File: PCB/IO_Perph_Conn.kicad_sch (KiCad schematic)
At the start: 18 parts, among them J2 Conn_02x06_Odd_Even, U4 STM32MP157FABx, Y601 NX2012SA-32.768K

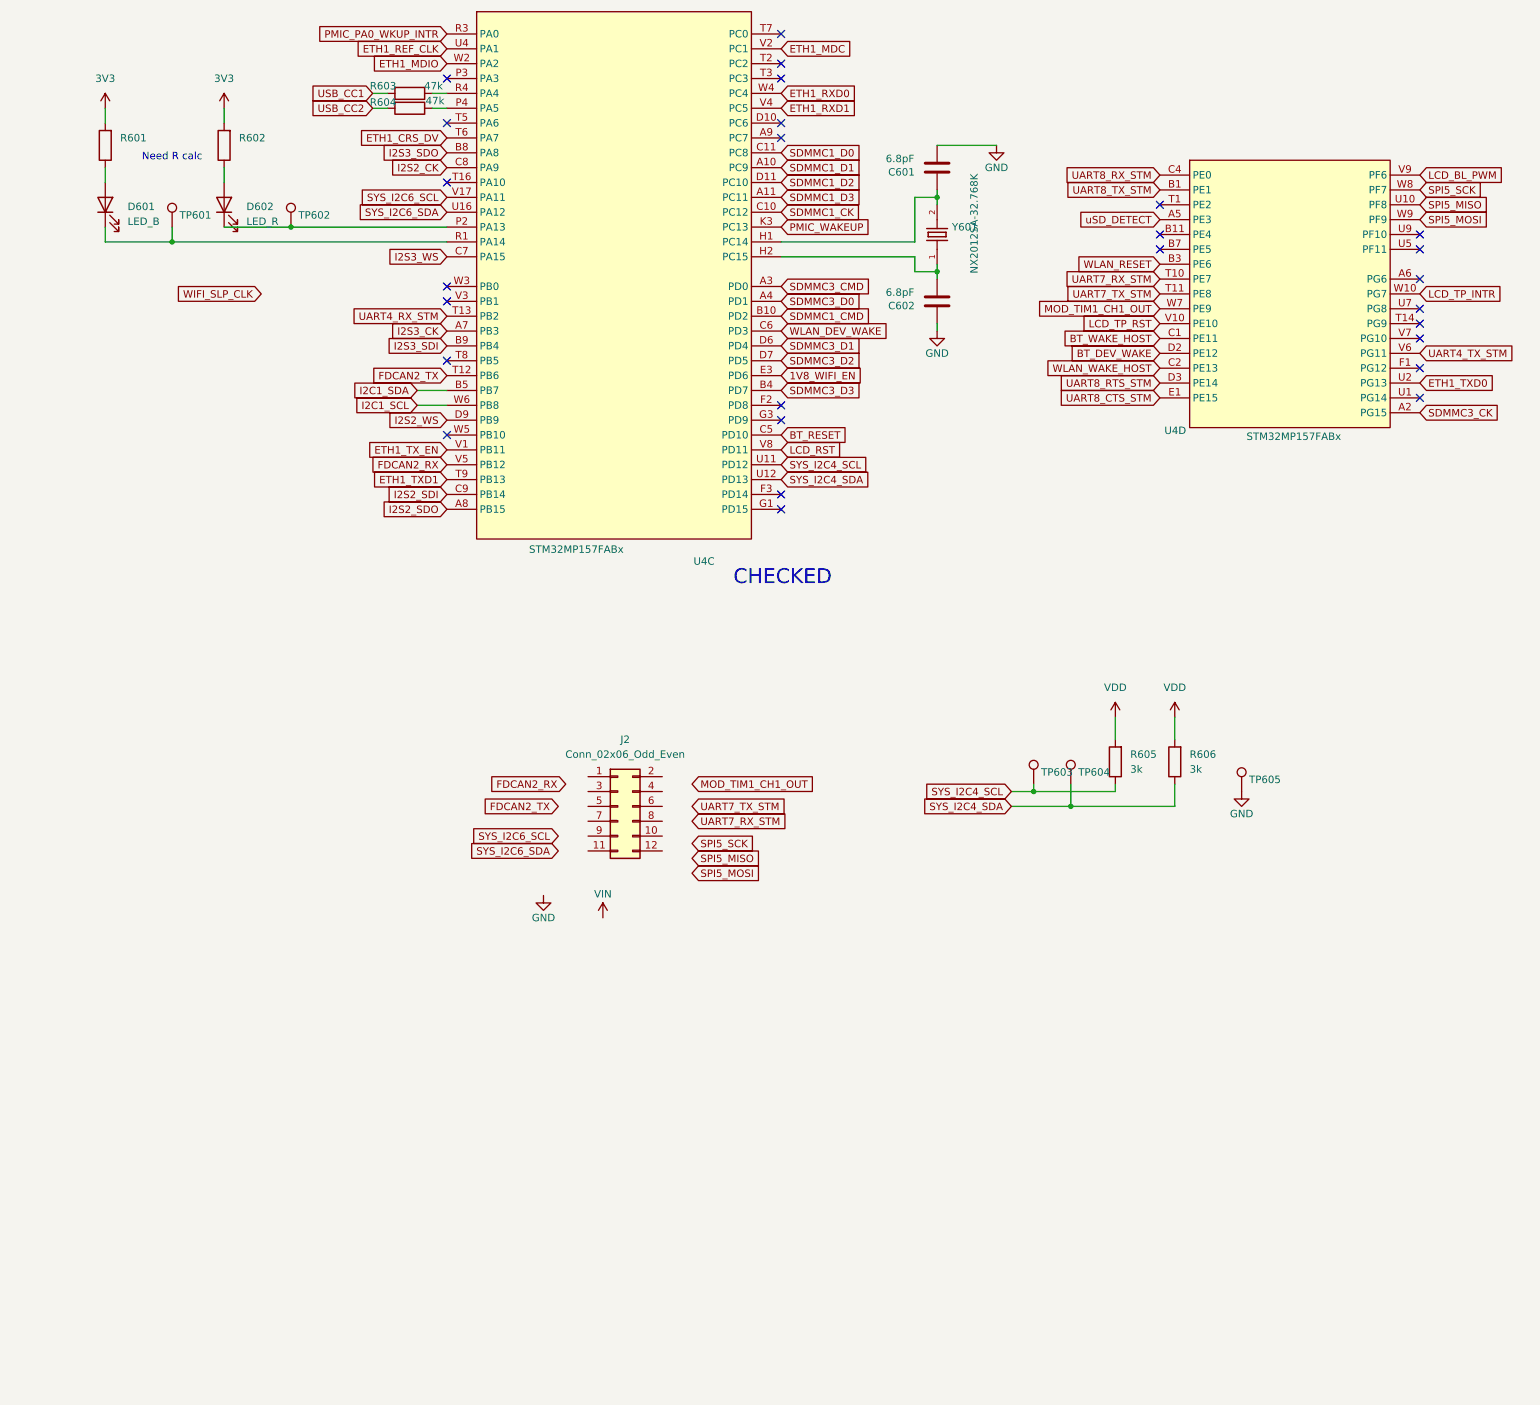
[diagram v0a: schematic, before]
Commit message: UPDATE
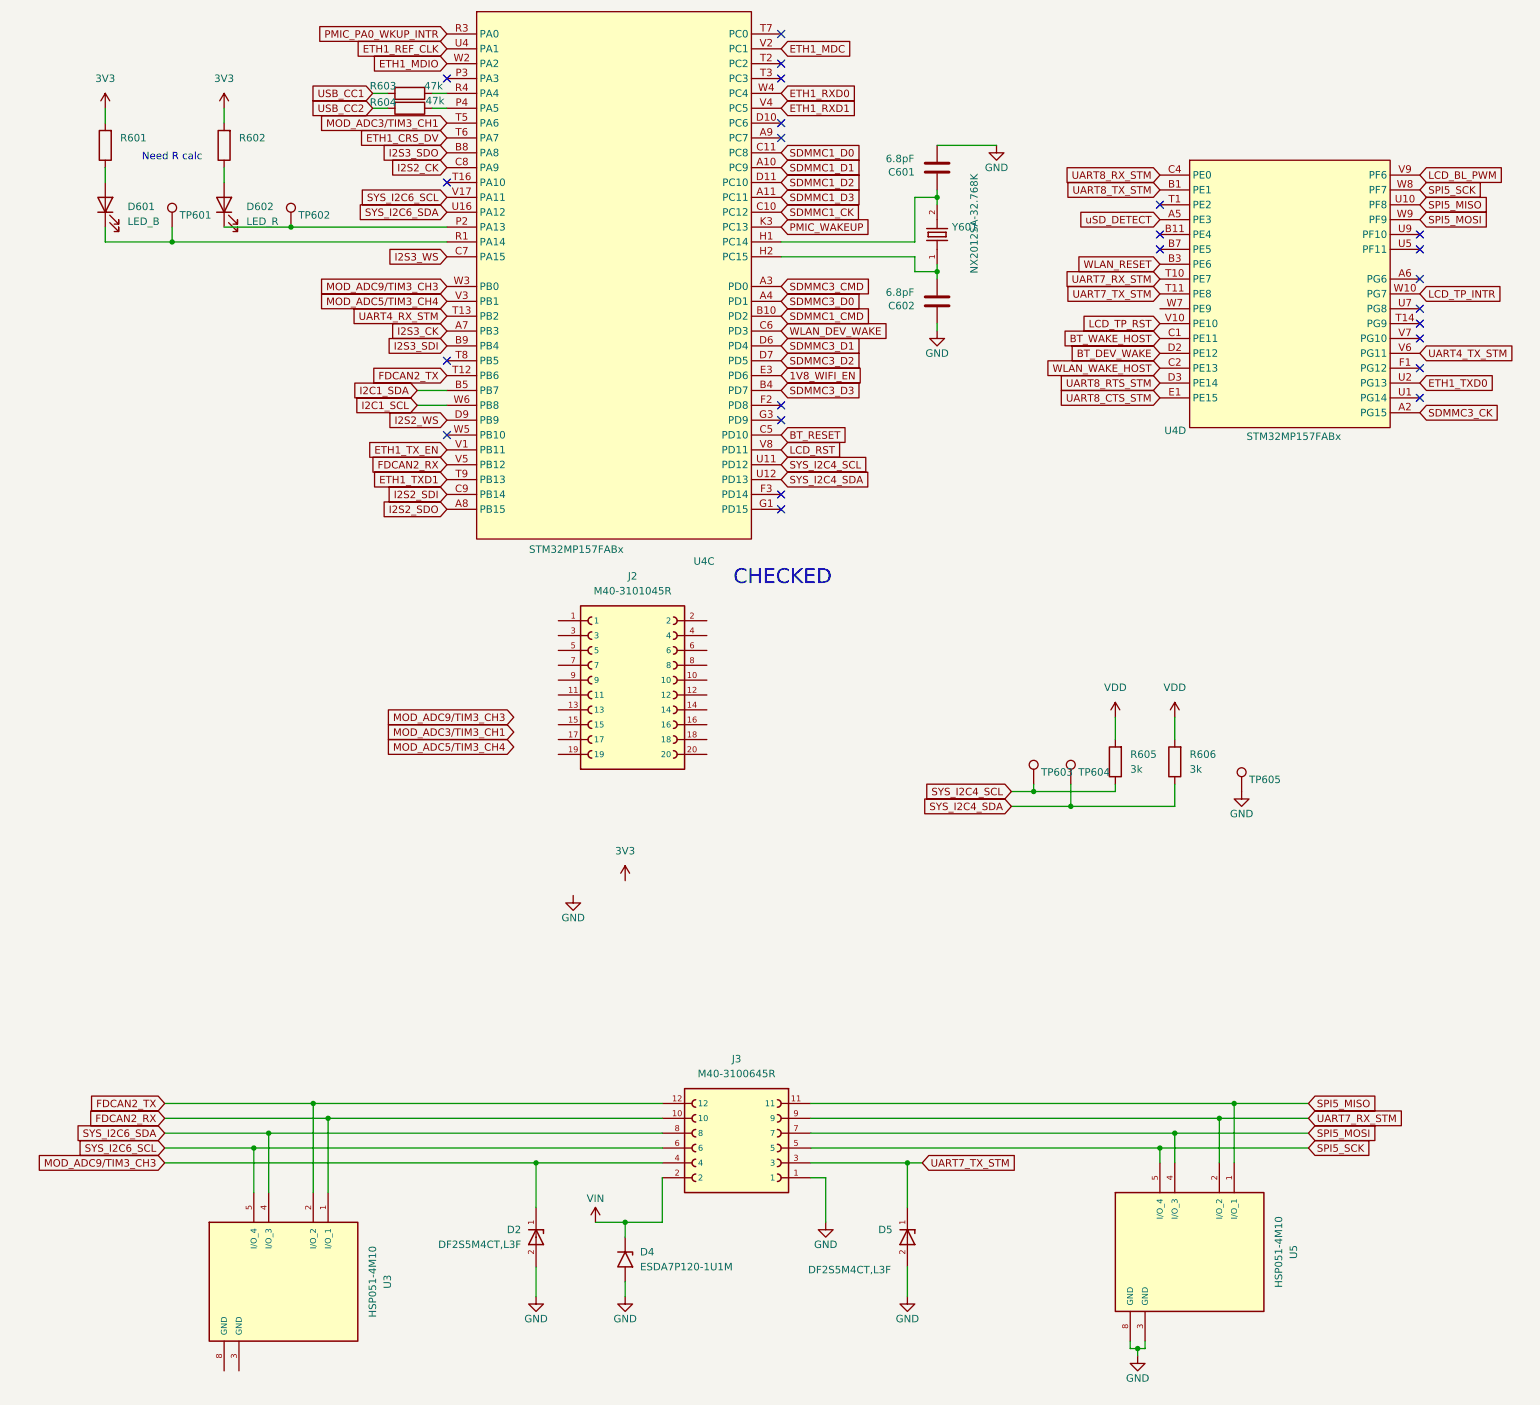
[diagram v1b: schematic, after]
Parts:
- removed J2: Conn_02x06_Odd_Even, Connector_PinHeader_1.00mm:PinHeader_2x06_P1.00mm_Vertical_SMD, symbol Connector_Generic:Conn_02x06_Odd_Even
- added D2, D5: DF2S5M4CT,L3F, Diode_SMD:D_SOD-882, symbol PTVS3V3S1UR:PTVS3V3S1UR
- added D4: ESDA7P120-1U1M, lib:DIODE_ESDA7P120-1U1M_STM, symbol Diode:SMAJ5.0A
- added J2: M40-3101045R, lib:HARWIN_M40-3101045R, symbol M40-3101045R:M40-3101045R
- added J3: M40-3100645R, lib:HARWIN_M40-3100645R, symbol M40-3100645R:M40-3100645R
- added U3, U5: HSP051-4M10, lib:IC_HSP051-4M10, symbol HSP051-4M10:HSP051-4M10
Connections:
- net FDCAN2_RX: now also J3.10, U3.1 (I/O_1), U3.10 (NC)
- net FDCAN2_TX: now also J3.12, U3.2 (I/O_2), U3.9 (NC)
- net GND: now also D2.2, D4.2 (A2), D5.2, J3.1, U5.3 (GND), U5.8 (GND)
- net SPI5_MISO: now also J3.11, U5.1 (I/O_1), U5.10 (NC)
- net SPI5_MOSI: now also J3.7, U5.4 (I/O_3), U5.7 (NC)
- net SPI5_SCK: now also J3.5, U5.5 (I/O_4), U5.6 (NC)
- net SYS_I2C6_SCL: now also J3.6, U3.5 (I/O_4), U3.6 (NC)
- net SYS_I2C6_SDA: now also J3.8, U3.4 (I/O_3), U3.7 (NC)
- net UART7_RX_STM: now also J3.9, U5.2 (I/O_2), U5.9 (NC)
- net UART7_TX_STM: now also D5.1, J3.3
- net VIN: now also D4.1 (A1), J3.2
- net MOD_ADC3/TIM3_CH1: now reaches U4.T5 (PA6)
- net MOD_ADC5/TIM3_CH4: now reaches U4.V3 (PB1)
- net MOD_ADC9/TIM3_CH3: now reaches U4.W3 (PB0)
- net MOD_ADC9/TIM3_CH3: now also D2.1, J3.4
- net MOD_TIM1_CH1_OUT: no longer names the net of U4.W7 (PE9)
- no-connect marks 27 -> 24

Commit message: UPDATE
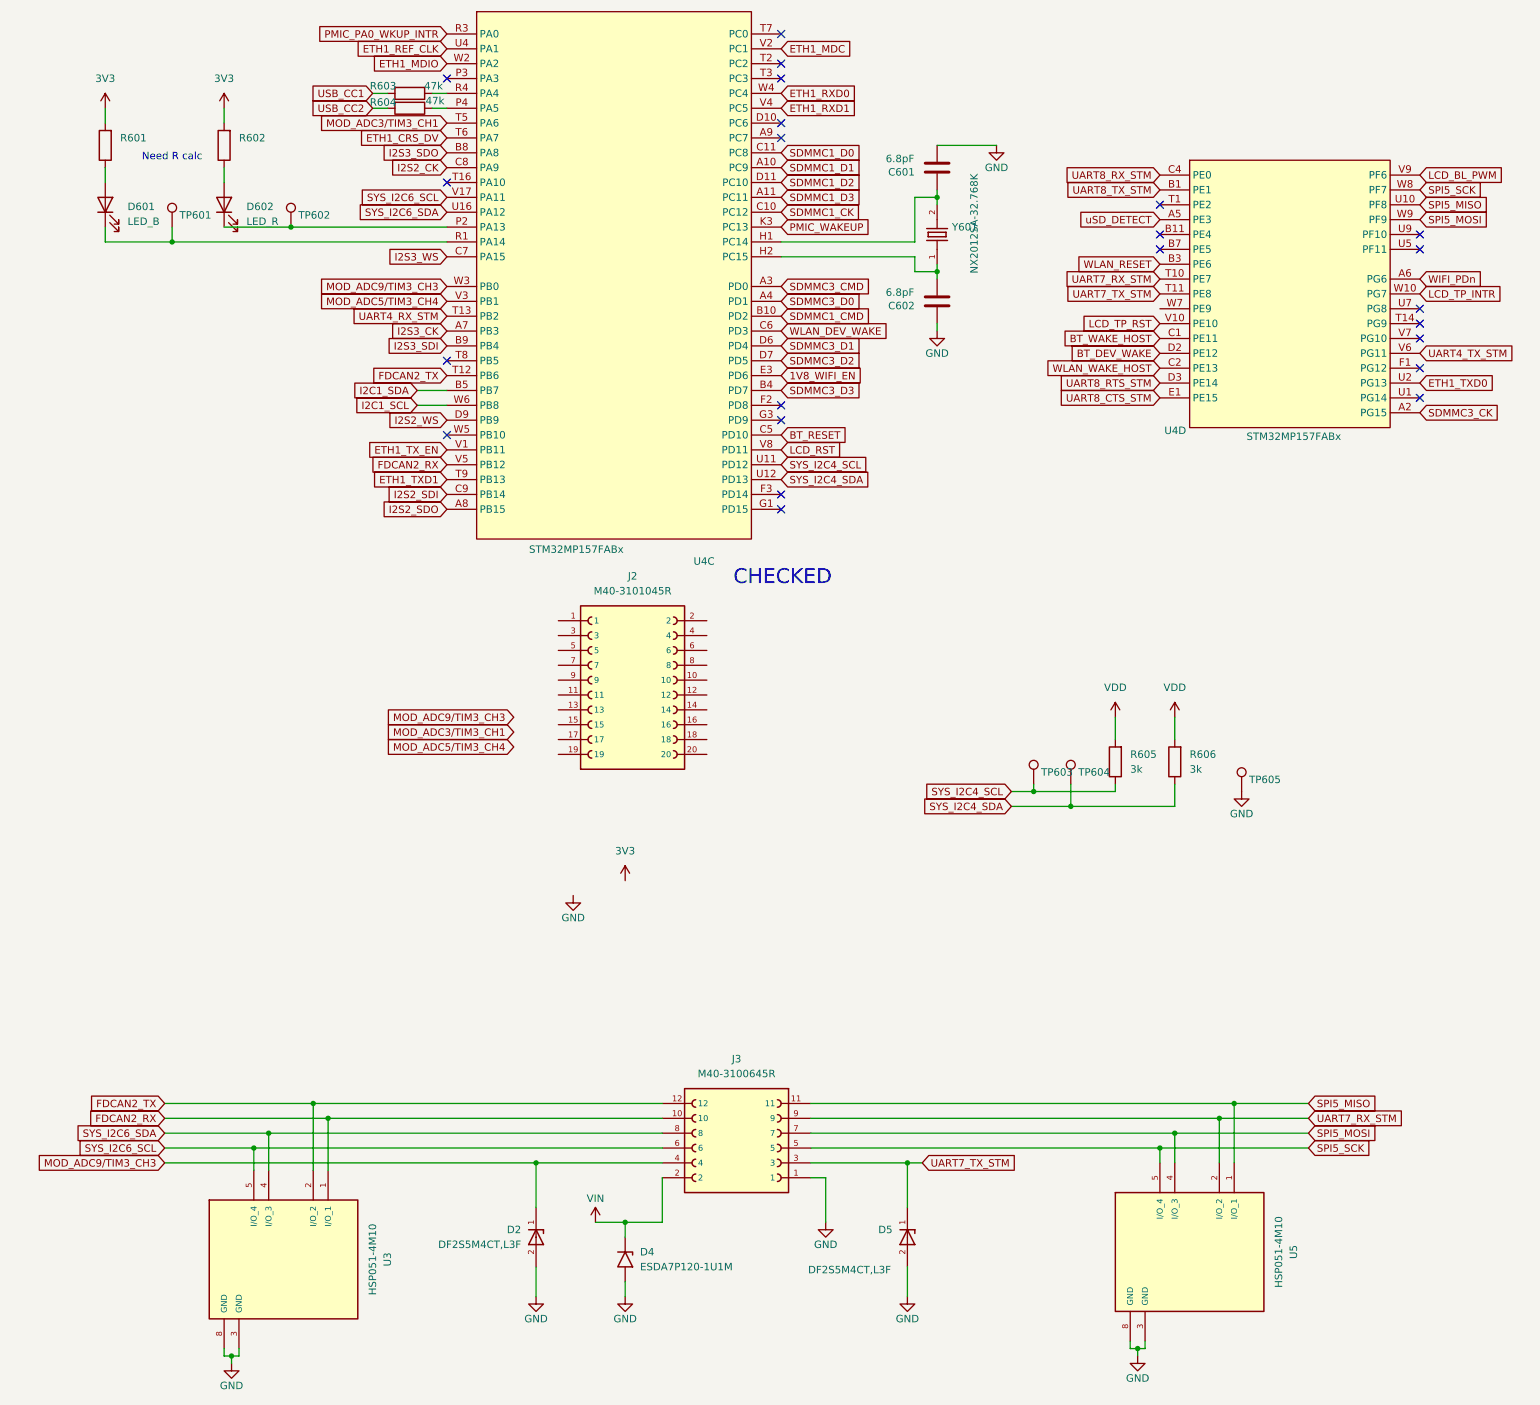
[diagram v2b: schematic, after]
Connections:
- net GND: now also U3.3 (GND), U3.8 (GND)
- net WIFI_PDn: now reaches U4.A6 (PG6)
- no-connect marks 24 -> 23
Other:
- moved on the sheet: U3
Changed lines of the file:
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@@
 	)
 	(junction
+		(at 68.58 276.86)
+		(diameter 0)
+		(color 0 0 0 0)
+	)
+	(junction
 		(at 237.49 236.22)
 		(diameter 0)
@@
 	)
 	(no_connect
-		(at 271.78 92.71)
-	)
-	(no_connect
 		(at 162.56 55.88)
 	)
@@
 	(wire
 		(pts
-			(xy 74.93 238.76) (xy 74.93 248.92)
+			(xy 74.93 238.76) (xy 74.93 245.11)
+		)
+		(stroke
+			(width 0)
+			(type default)
+		)
+	)
+	(wire
+		(pts
+			(xy 67.31 276.86) (xy 68.58 276.86)
 		)
 		(stroke
@@
 	(wire
 		(pts
+			(xy 67.31 275.59) (xy 67.31 276.86)
+		)
+		(stroke
+			(width 0)
+			(type default)
+		)
+	)
+	(wire
+		(pts
 			(xy 46.99 73.66) (xy 46.99 76.2)
 		)
@@
 	(wire
 		(pts
-			(xy 82.55 233.68) (xy 82.55 248.92)
+			(xy 82.55 233.68) (xy 82.55 245.11)
 		)
 		(stroke
@@
 	(wire
 		(pts
+			(xy 69.85 276.86) (xy 69.85 275.59)
+		)
+		(stroke
+			(width 0)
+			(type default)
+		)
+	)
+	(wire
+		(pts
 			(xy 201.93 182.88) (xy 212.09 182.88)
 		)
@@
 	(wire
 		(pts
+			(xy 68.58 278.13) (xy 68.58 276.86)
+		)
+		(stroke
+			(width 0)
+			(type default)
+		)
+	)
+	(wire
+		(pts
 			(xy 57.15 233.68) (xy 82.55 233.68)
 		)
@@
 	(wire
 		(pts
+			(xy 68.58 276.86) (xy 69.85 276.86)
+		)
+		(stroke
+			(width 0)
+			(type default)
+		)
+	)
+	(wire
+		(pts
 			(xy 162.56 88.9) (xy 185.42 88.9)
 		)
@@
 	(wire
 		(pts
-			(xy 72.39 241.3) (xy 72.39 248.92)
+			(xy 72.39 241.3) (xy 72.39 245.11)
 		)
 		(stroke
@@
 	(wire
 		(pts
-			(xy 85.09 236.22) (xy 85.09 248.92)
+			(xy 85.09 236.22) (xy 85.09 245.11)
 		)
 		(stroke
@@
 		)
 	)
+	(global_label "WIFI_PDn"
+		(shape input)
+		(at 271.78 92.71 0)
+		(fields_autoplaced yes)
+		(effects
+			(font
+				(size 1.27 1.27)
+			)
+			(justify left)
+		)
+		(property "Intersheetrefs" "${INTERSHEET_REFS}"
+			(at 283.1714 92.71 0)
+			(effects
+				(font
+					(size 1.27 1.27)
+				)
+				(justify left)
+				(hide yes)
+			)
+		)
+	)
 	(global_label "UART7_RX_STM"
 		(shape input)
@@
 	(symbol
 		(lib_id "HSP051-4M10:HSP051-4M10")
-		(at 77.47 264.16 270)
+		(at 77.47 260.35 270)
 		(unit 1)
 		(exclude_from_sim no)
@@
 		(dnp no)
 		(property "Reference" "U3"
-			(at 95.25 264.16 0)
+			(at 95.25 260.35 0)
 			(effects
 				(font
@@
 		)
 		(property "Value" "HSP051-4M10"
-			(at 92.71 264.16 0)
+			(at 92.71 260.35 0)
 			(effects
 				(font
@@
 		)
 		(property "Footprint" "lib:IC_HSP051-4M10"
-			(at 77.47 264.16 0)
+			(at 77.47 260.35 0)
 			(effects
 				(font
@@
 		)
 		(property "Datasheet" ""
-			(at 77.47 264.16 0)
+			(at 77.47 260.35 0)
 			(effects
 				(font
@@
 		)
 		(property "Description" ""
-			(at 77.47 264.16 0)
+			(at 77.47 260.35 0)
 			(effects
 				(font
@@
 		)
 		(property "MF" "STMicroelectronics"
-			(at 77.47 264.16 0)
+			(at 77.47 260.35 0)
 			(effects
 				(font
@@
 		)
 		(property "MAXIMUM_PACKAGE_HEIGHT" "0.5mm"
-			(at 77.47 264.16 0)
+			(at 77.47 260.35 0)
 			(effects
 				(font
@@
 		)
 		(property "Package" "UQFN-10 STMicroelectronics"
-			(at 77.47 264.16 0)
+			(at 77.47 260.35 0)
 			(effects
 				(font
@@
 		)
 		(property "Description_1" "10V Clamp 1A (8/20µs) Ipp Tvs Diode Surface Mount 10-UQFN (2.5x1)"
-			(at 77.47 264.16 0)
+			(at 77.47 260.35 0)
 			(effects
 				(font
@@
 		)
 		(property "MANUFACTURER" "STMicroelectronics"
-			(at 77.47 264.16 0)
+			(at 77.47 260.35 0)
 			(effects
 				(font
@@
 		)
 		(property "Mouser P/N" "511-HSP051-4M10"
-			(at 77.47 264.16 0)
+			(at 77.47 260.35 0)
 			(effects
 				(font
@@
 		)
 		(property "BUILT_BY" ""
-			(at 77.47 264.16 0)
+			(at 77.47 260.35 0)
 			(effects
 				(font
@@
 		)
 		(property "COPYRIGHT" ""
-			(at 77.47 264.16 0)
+			(at 77.47 260.35 0)
 			(effects
 				(font
@@
 		)
 		(property "LCSC Part #" "C1973641"
-			(at 77.47 264.16 0)
+			(at 77.47 260.35 0)
 			(effects
 				(font
@@
 		)
 		(property "MANUFACTURER_PART_NUMBER" ""
-			(at 77.47 264.16 0)
+			(at 77.47 260.35 0)
 			(effects
 				(font
@@
 		)
 		(property "SNAPEDA_PN" ""
-			(at 77.47 264.16 0)
+			(at 77.47 260.35 0)
 			(effects
 				(font
@@
 		)
 		(property "SOURCELIBRARY" ""
-			(at 77.47 264.16 0)
+			(at 77.47 260.35 0)
 			(effects
 				(font
@@
 		)
 		(property "VENDOR" ""
-			(at 77.47 264.16 0)
+			(at 77.47 260.35 0)
 			(effects
 				(font
@@
 		)
 		(property "REC P/N" " HSP051-4M10"
-			(at 77.47 264.16 0)
+			(at 77.47 260.35 0)
 			(effects
 				(font
@@
 					(unit 1)
 				)
+			)
+		)
+	)
+	(symbol
+		(lib_id "power:GND")
+		(at 68.58 278.13 0)
+		(unit 1)
+		(exclude_from_sim no)
+		(in_bom yes)
+		(on_board yes)
+		(dnp no)
+		(property "Reference" "#PWR028"
+			(at 68.58 284.48 0)
+			(effects
+				(font
+					(size 1.27 1.27)
+				)
+				(hide yes)
+			)
+		)
+		(property "Value" "GND"
+			(at 68.58 281.94 0)
+			(effects
+				(font
+					(size 1.27 1.27)
+				)
+			)
+		)
+		(property "Footprint" ""
+			(at 68.58 278.13 0)
+			(effects
+				(font
+					(size 1.27 1.27)
+				)
+				(hide yes)
+			)
+		)
+		(property "Datasheet" ""
+			(at 68.58 278.13 0)
+			(effects
+				(font
+					(size 1.27 1.27)
+				)
+				(hide yes)
+			)
+		)
+		(property "Description" "Power symbol creates a global label with name \"GND\" , ground"
+			(at 68.58 278.13 0)
+			(effects
+				(font
+					(size 1.27 1.27)
+				)
+				(hide yes)
+			)
+		)
+		(pin "1"
+		)
+		(instances
+			(project "MPU_MOD"
+				(path "/65890f61-d586-475b-928a-b635a5e4e59e/fb3927f9-2e38-40e3-962e-323526569853"
+					(reference "#PWR028")
+					(unit 1)
+				)
